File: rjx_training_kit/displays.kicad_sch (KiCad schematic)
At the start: 30 parts, among them Q1 BC817, Q2 BC808, Q3 BC808, Q4 BC808, Q5 BC808, Q6 BC808, U4 LTC-4627JD (Red)

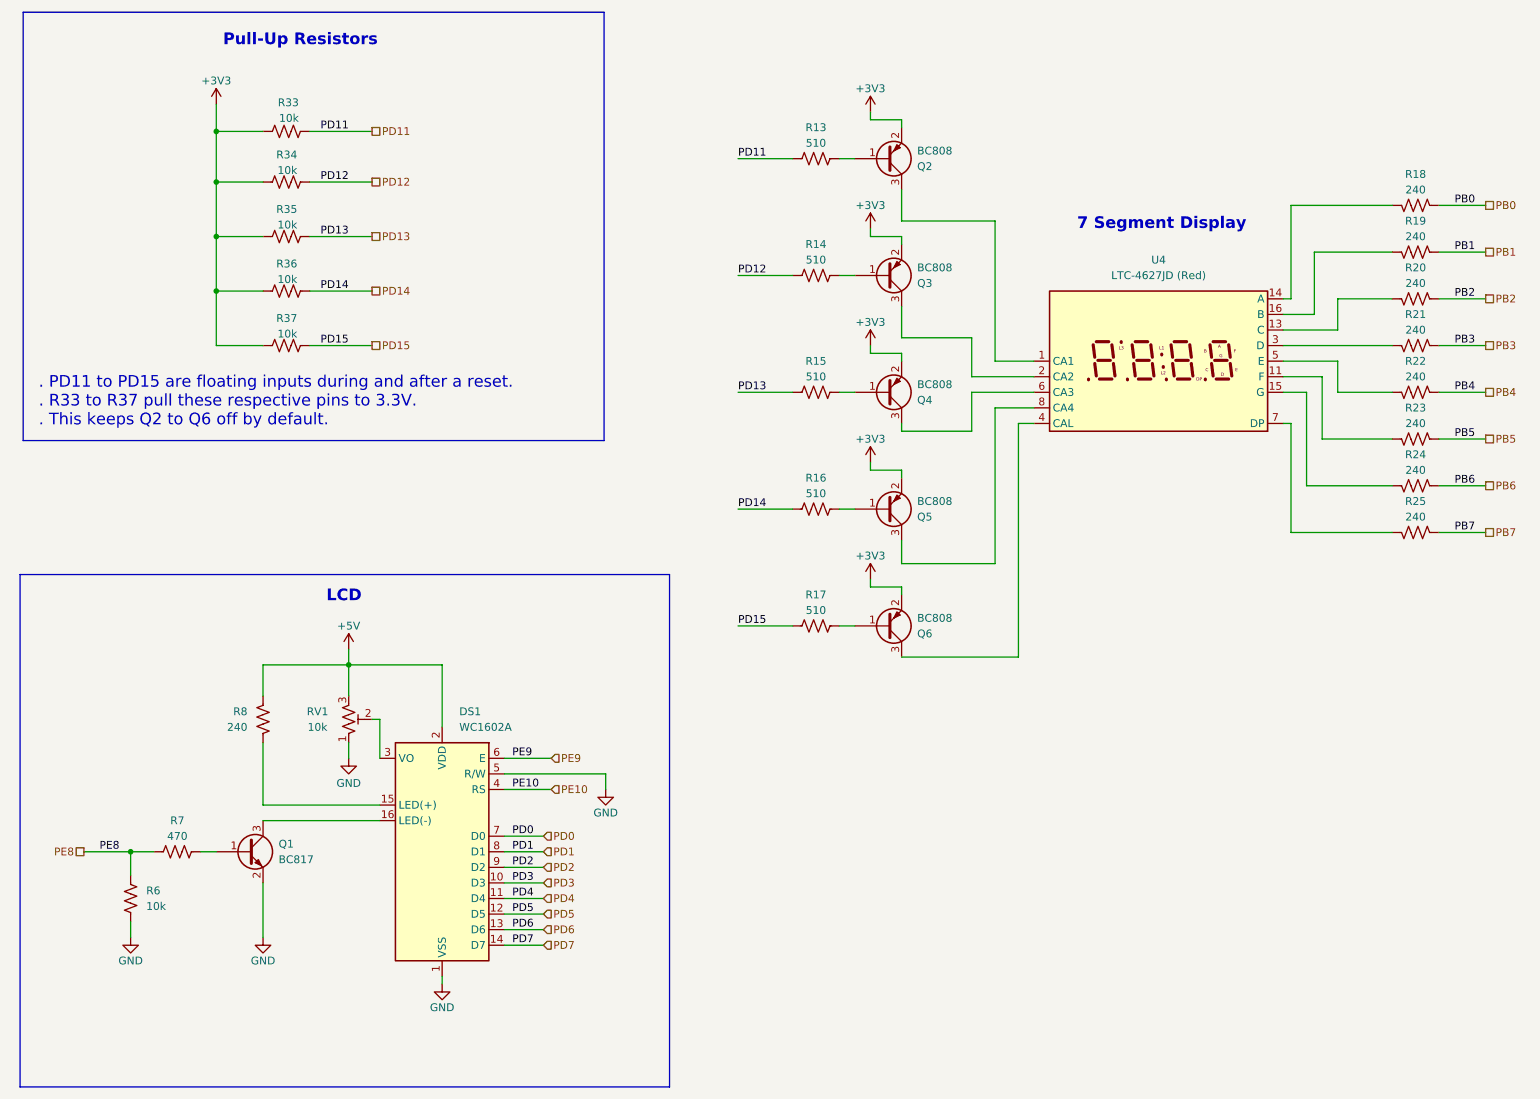
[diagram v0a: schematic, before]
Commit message: Update
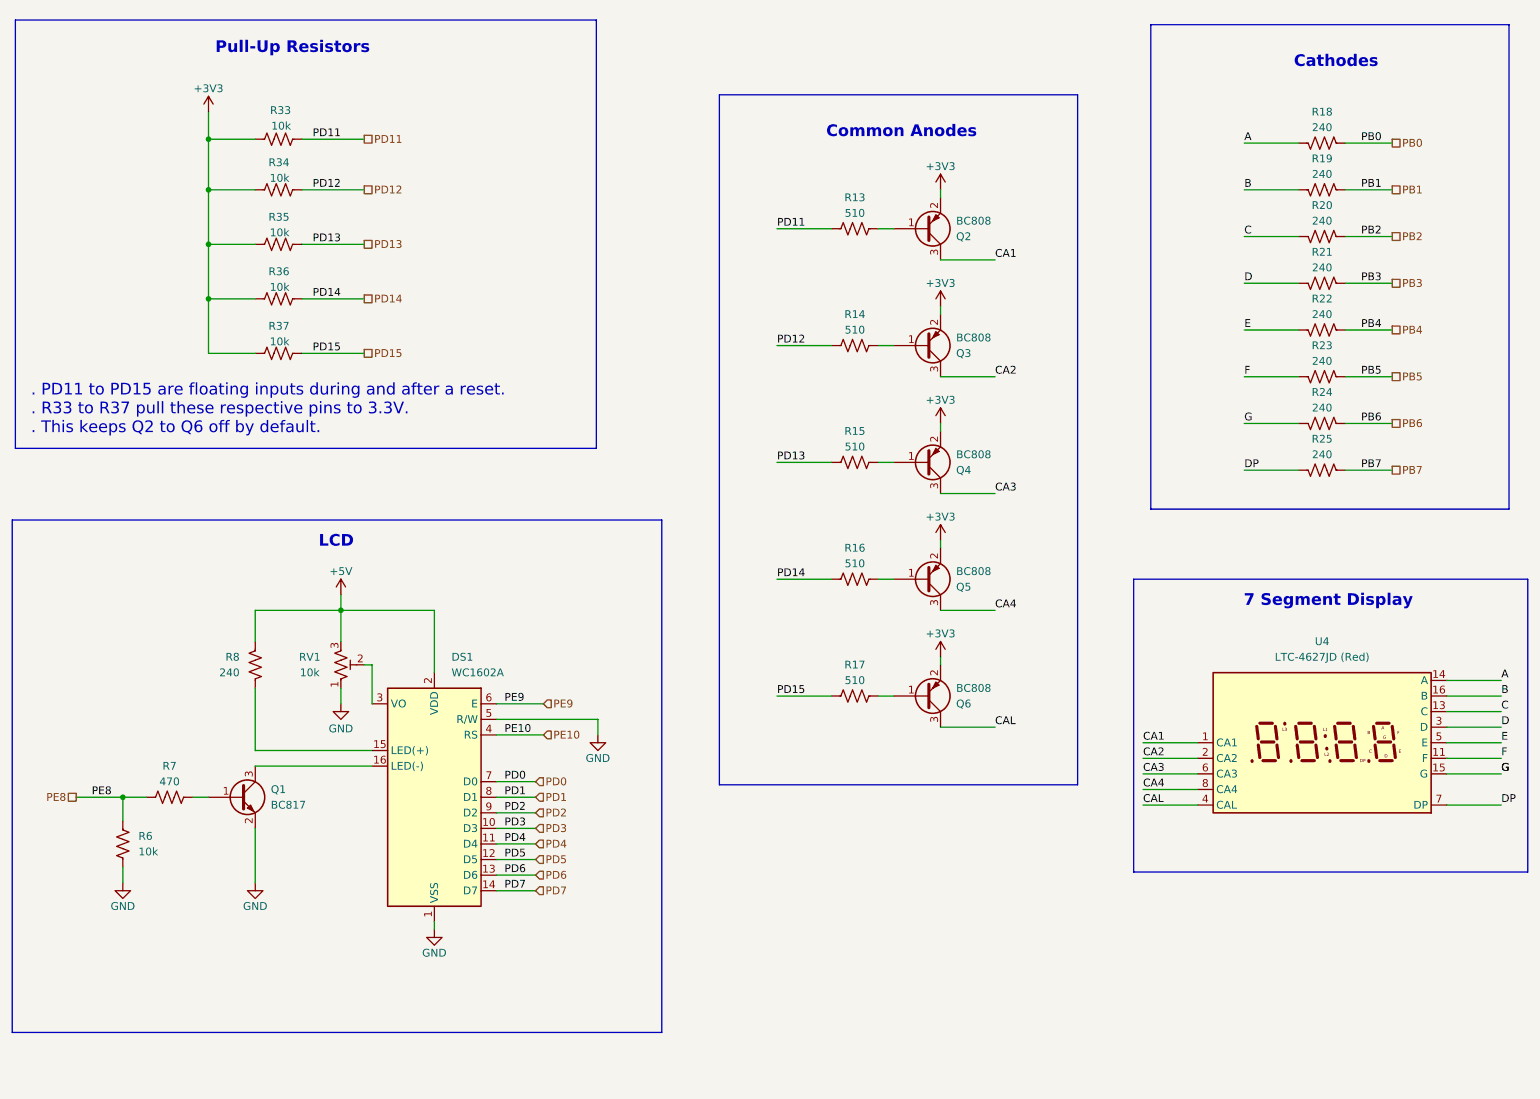
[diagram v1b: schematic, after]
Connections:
- net B: now reaches R19.2, U4.16 (B)
- net CA2: now reaches Q3.3 (C), U4.2 (CA2)
- net C: now reaches R20.2, U4.13 (C)
- net CA4: now reaches Q5.3 (C), U4.8 (CA4)
- net F: now reaches R23.2, U4.11 (F)
- net CA3: now reaches Q4.3 (C), U4.6 (CA3)
- net G: now reaches R24.2, U4.15 (G)
- net CA1: now reaches Q2.3 (C), U4.1 (CA1)
- net DP: now reaches R25.2, U4.7 (DP)
- net D: now reaches R21.2, U4.3 (D)
- net E: now reaches R22.2, U4.5 (E)
- net CAL: now reaches Q6.3 (C), U4.4 (CAL)
- net A: now reaches R18.2, U4.14 (A)
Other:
- note added: "Cathodes"
- note added: "Common Anodes"
- moved on the sheet: DS1, Q1, Q2, Q3, Q4, Q5, Q6, R13, R14, R15, R16, R17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
